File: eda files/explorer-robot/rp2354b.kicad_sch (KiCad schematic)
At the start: 34 parts, among them J1 DBG, SW1 SW_Push, U1 RP2354B, U2 AMS1117-3.3, Y1 ABM8-272-T3

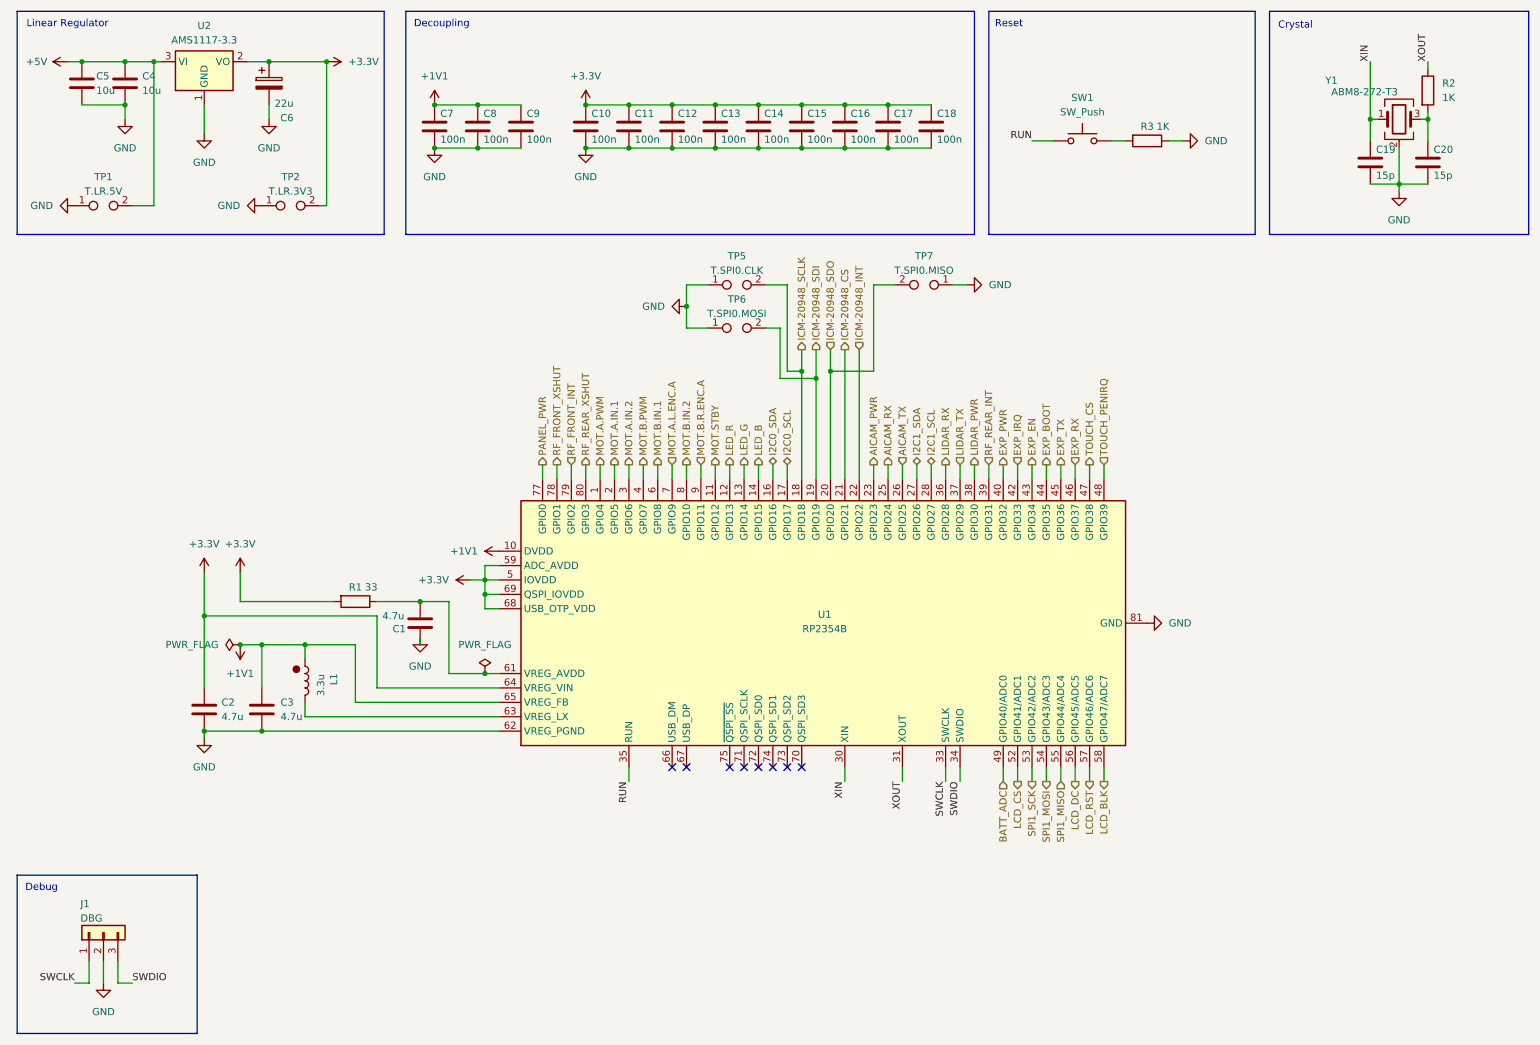
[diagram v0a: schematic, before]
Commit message: place test points, tidy up, ERC
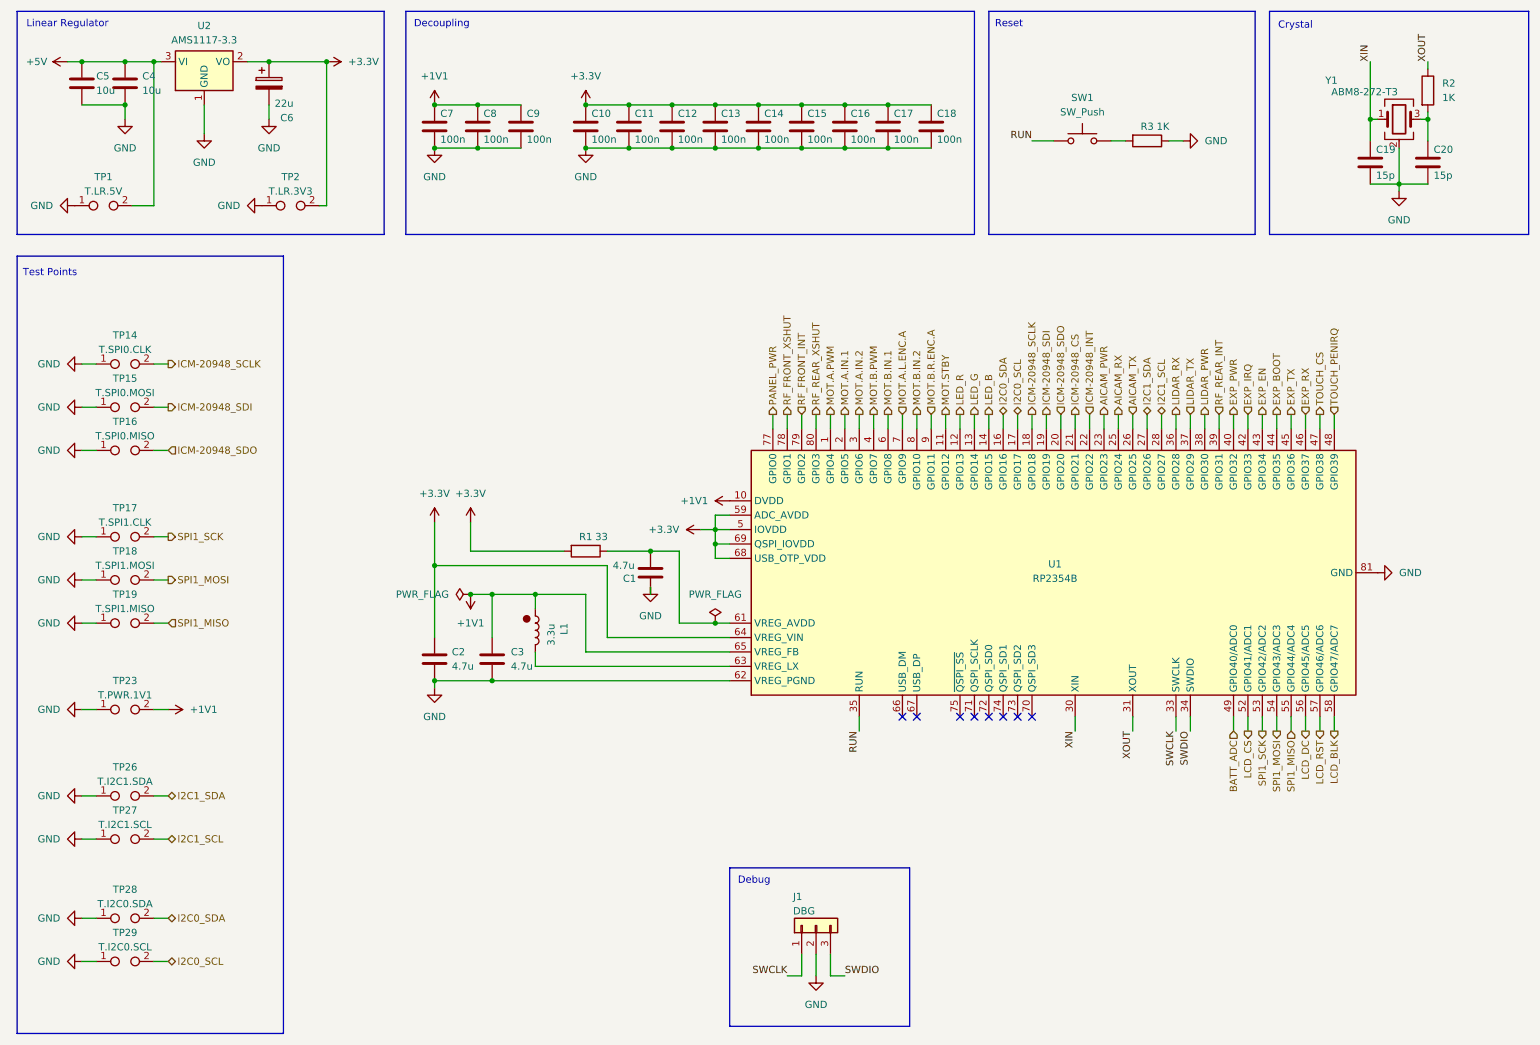
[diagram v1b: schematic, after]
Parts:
- removed TP5: T.SPI0.CLK, tp:TestPoint_Bridge_Pitch3.81mm_Drill1.3mm, symbol Connector:TestPoint_2Pole
- removed TP6: T.SPI0.MOSI, tp:TestPoint_Bridge_Pitch3.81mm_Drill1.3mm, symbol Connector:TestPoint_2Pole
- removed TP7: T.SPI0.MISO, tp:TestPoint_Bridge_Pitch3.81mm_Drill1.3mm, symbol Connector:TestPoint_2Pole
- added TP14: T.SPI0.CLK, Connector_PinHeader_2.54mm:PinHeader_1x02_P2.54mm_Vertical, symbol Connector:TestPoint_2Pole
- added TP15: T.SPI0.MOSI, Connector_PinHeader_2.54mm:PinHeader_1x02_P2.54mm_Vertical, symbol Connector:TestPoint_2Pole
- added TP16: T.SPI0.MISO, Connector_PinHeader_2.54mm:PinHeader_1x02_P2.54mm_Vertical, symbol Connector:TestPoint_2Pole
- added TP17: T.SPI1.CLK, Connector_PinHeader_2.54mm:PinHeader_1x02_P2.54mm_Vertical, symbol Connector:TestPoint_2Pole
- added TP18: T.SPI1.MOSI, Connector_PinHeader_2.54mm:PinHeader_1x02_P2.54mm_Vertical, symbol Connector:TestPoint_2Pole
- added TP19: T.SPI1.MISO, Connector_PinHeader_2.54mm:PinHeader_1x02_P2.54mm_Vertical, symbol Connector:TestPoint_2Pole
- added TP23: T.PWR.1V1, Connector_PinHeader_2.54mm:PinHeader_1x02_P2.54mm_Vertical, symbol Connector:TestPoint_2Pole
- added TP26: T.I2C1.SDA, Connector_PinHeader_2.54mm:PinHeader_1x02_P2.54mm_Vertical, symbol Connector:TestPoint_2Pole
- added TP27: T.I2C1.SCL, Connector_PinHeader_2.54mm:PinHeader_1x02_P2.54mm_Vertical, symbol Connector:TestPoint_2Pole
- added TP28: T.I2C0.SDA, Connector_PinHeader_2.54mm:PinHeader_1x02_P2.54mm_Vertical, symbol Connector:TestPoint_2Pole
- added TP29: T.I2C0.SCL, Connector_PinHeader_2.54mm:PinHeader_1x02_P2.54mm_Vertical, symbol Connector:TestPoint_2Pole
- TP1, TP2: footprint tp:TestPoint_Bridge_Pitch3.81mm_Drill1.3mm -> Connector_PinHeader_2.54mm:PinHeader_1x02_P2.54mm_Vertical
- Y1: footprint Crystal:Crystal_SMD_Abracon_ABM8AIG-4Pin_3.2x2.5mm -> easyeda imports:CRYSTAL-SMD_4P-L3.2-W2.5-BL
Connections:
- net +1V1: now also TP23.2
- net GND: now also TP14.1, TP15.1, TP16.1, TP17.1, TP18.1, TP19.1, TP23.1, TP26.1, TP27.1, TP28.1, TP29.1
- net I2C0_SCL: now also TP29.2
- net I2C0_SDA: now also TP28.2
- net I2C1_SCL: now also TP27.2
- net I2C1_SDA: now also TP26.2
- net ICM-20948_SCLK: now also TP14.2
- net ICM-20948_SDI: now also TP15.2
- net ICM-20948_SDO: now also TP16.2
- net SPI1_MISO: now also TP19.2
- net SPI1_MOSI: now also TP18.2
- net SPI1_SCK: now also TP17.2
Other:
- note added: "Test Points"
- moved on the sheet: C1, C2, C3, J1, L1, R1, U1
